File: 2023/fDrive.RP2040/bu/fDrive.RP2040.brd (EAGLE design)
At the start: 68 x 58 mm, 11 parts

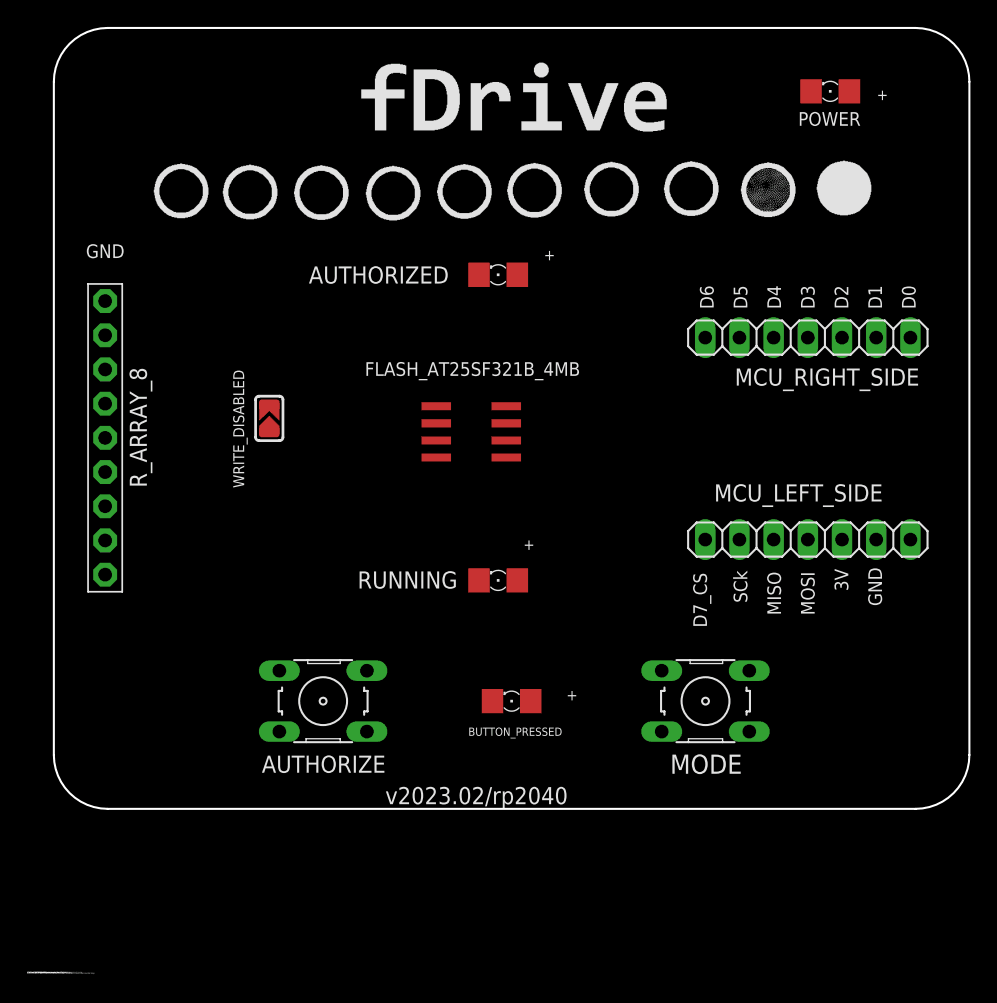
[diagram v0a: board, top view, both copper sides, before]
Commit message: fDrive update
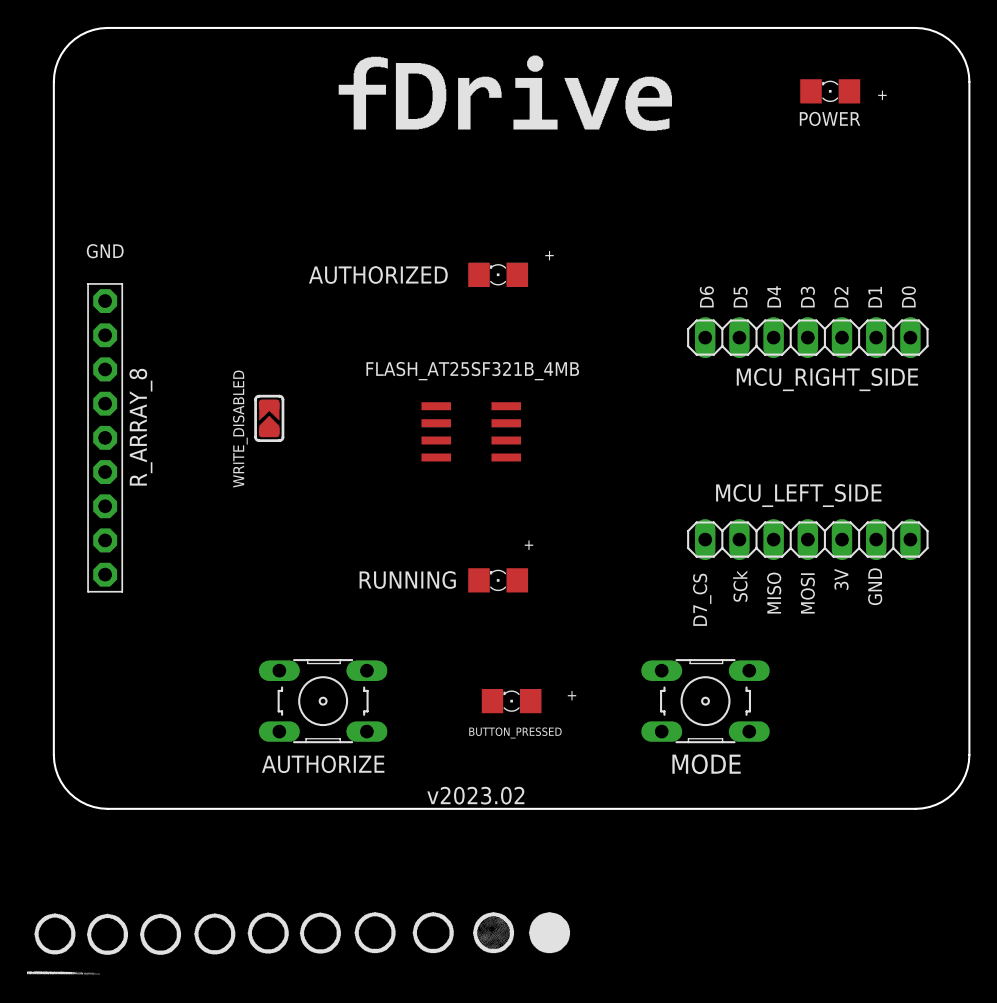
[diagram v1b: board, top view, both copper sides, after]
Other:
- board text added: "C:/DVT/Fred.PCB/2023/fDrive.RP2040/MadeInTheUSB.Logo.Gray.bmp"
- board text added: "v2023.02"
- board text removed: "v2023.02/rp2040"

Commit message: update
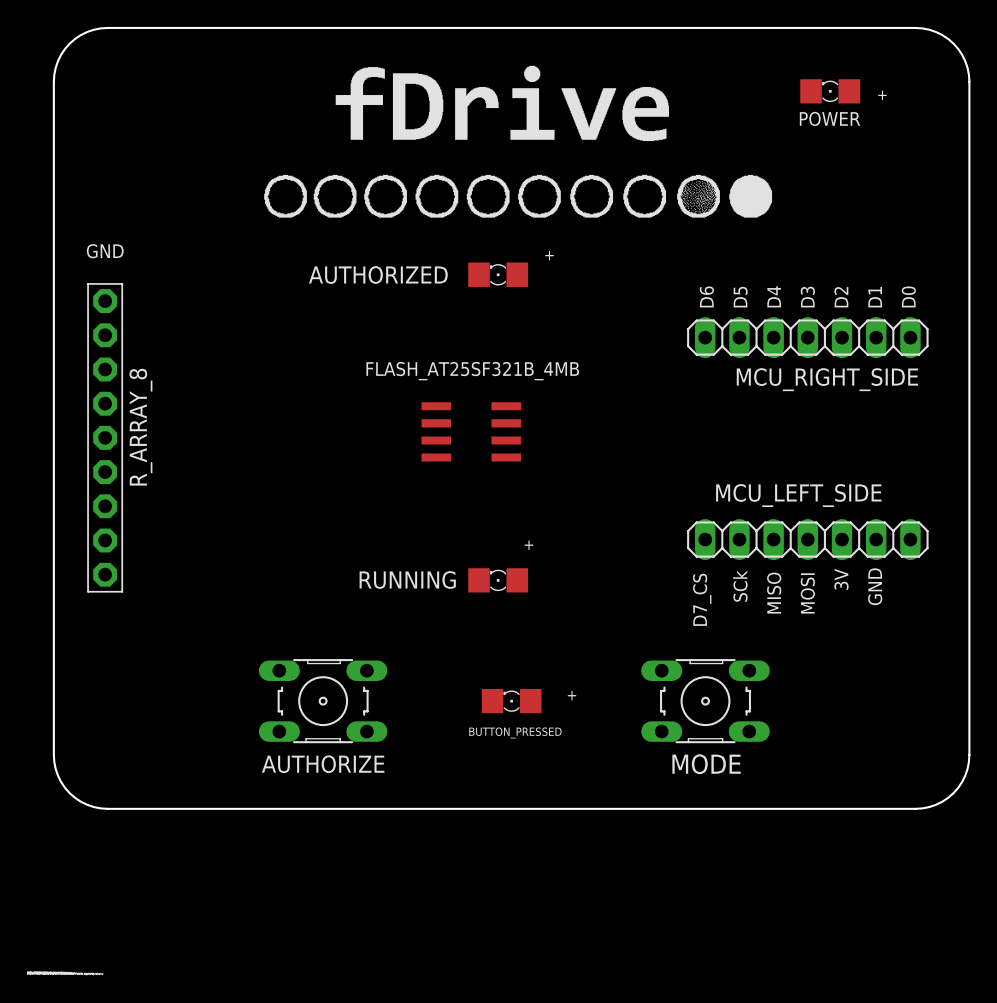
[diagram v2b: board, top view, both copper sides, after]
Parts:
- removed WRITE_DISABLED: (no value), microbuilder:SOLDERJUMPER_ARROW_NOPASTE
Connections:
- removed net MCU_VCC_5V: MCU_LEFT_SIDE.7
- removed net WP: FLASH_AT25SF321B_4MB.3, WRITE_DISABLED.2
- net GND: no longer WRITE_DISABLED.1
- net VCC_33: now also FLASH_AT25SF321B_4MB.3
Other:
- board text added: "C:/DVT/Fred.PCB/2023/fDrive.RP2040/MadeInTheUSB.Logo.Gray.50.bmp"
- board text removed: "v2023.02"
